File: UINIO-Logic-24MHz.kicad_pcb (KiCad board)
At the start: 2 copper layers, 48.8 x 25.5 mm, 51 parts, among them J1 Conn_01x10_Male, U1 AT24CS64-XHM, U2 74HC245C, U3 ME6211C33M5G-N, U4 CY7C68013A-56LTX, Y1 24MHz

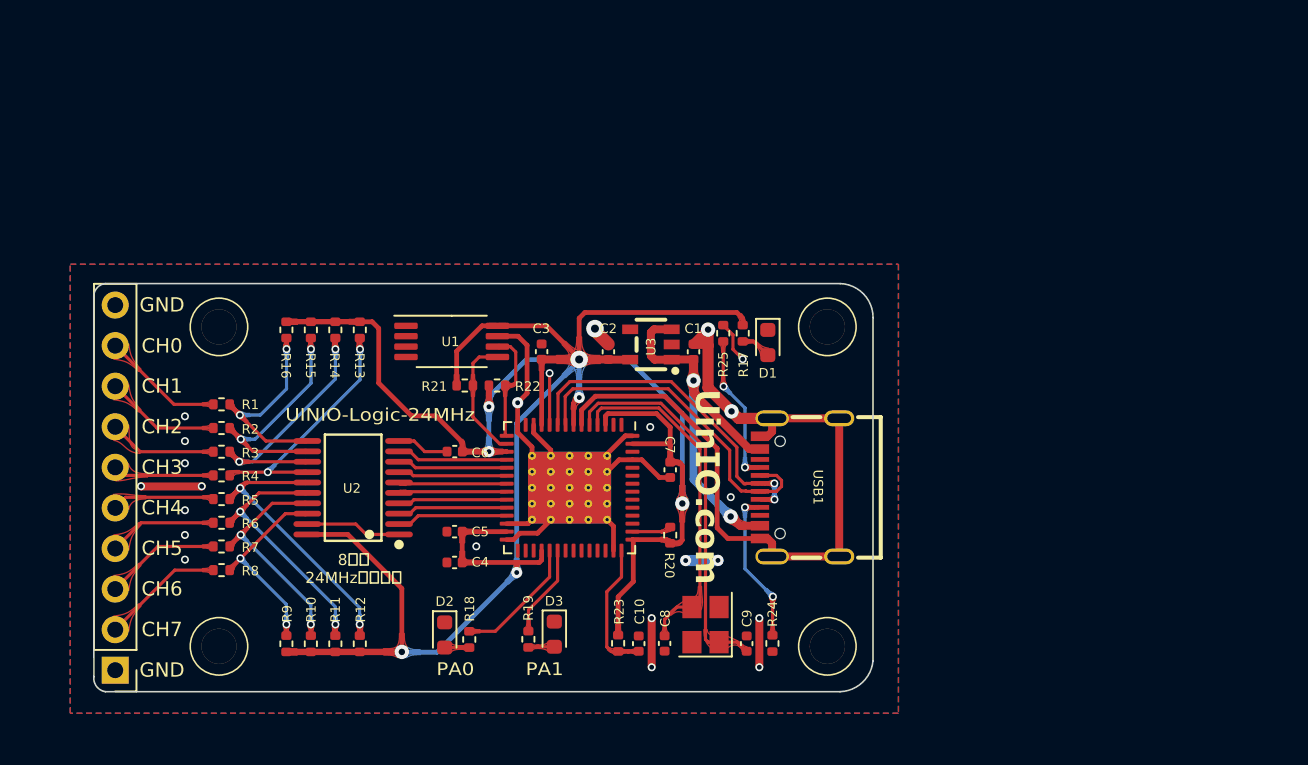
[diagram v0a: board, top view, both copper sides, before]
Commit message: Prepare version 3.1.0.
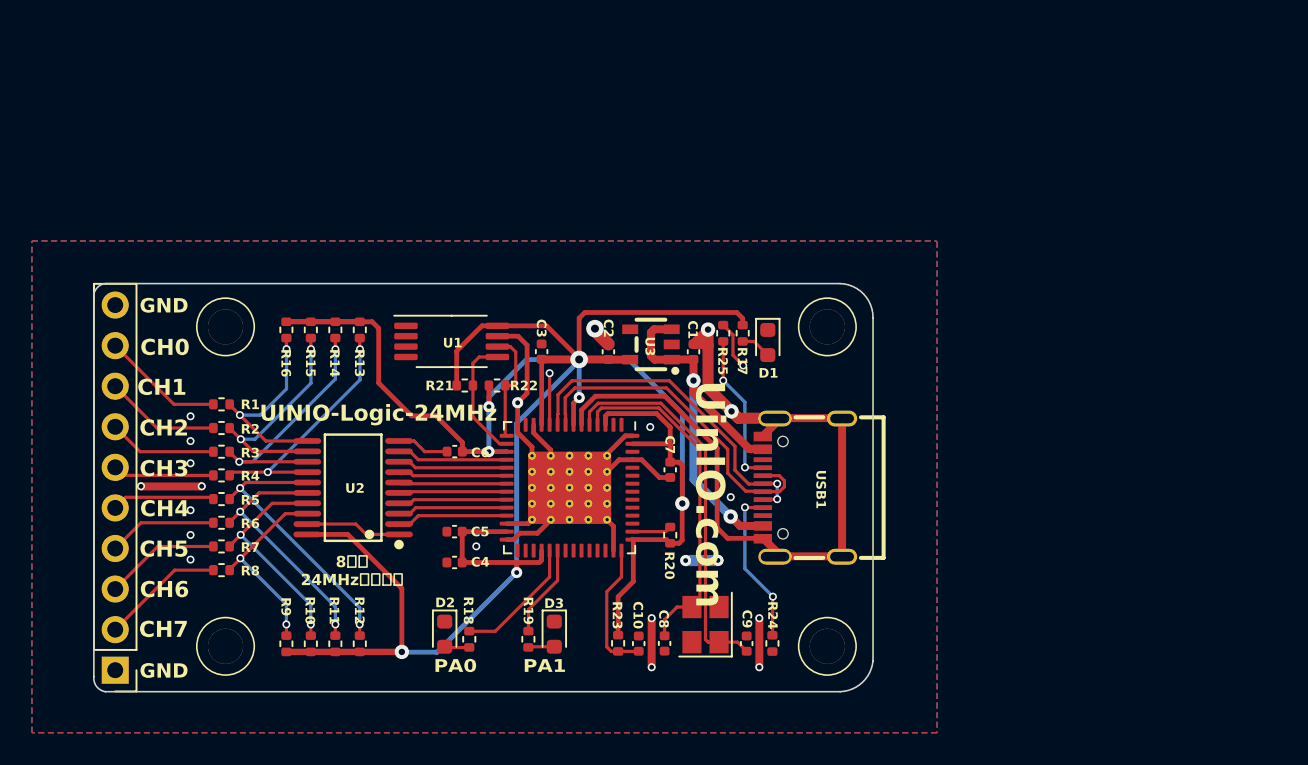
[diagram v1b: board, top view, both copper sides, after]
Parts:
- removed the ? at (144.7, 118.7)
- removed the ? at (130.6, 118.6)
- added ?: LOGO, LOGO, B.Cu at (136.1, 118.8)
- added ?: LOGO, LOGO, B.Cu at (120.4, 118.8)
- J1: value Conn_01x10_Male -> Conn_01x10_Pin
- moved HOLE1 0.41 mm to (114.5, 108.7)
- moved HOLE2 0.41 mm to (114.5, 128.7)
- moved USB1 0.18 mm to (150.6, 118.8)
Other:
- board text added: "UinIO.com"
- board text added: "Version 3.1.0"
- board text removed: "Version 3.0.0"

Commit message: Release UINIO-Logic-24MHz version 3.1.0.
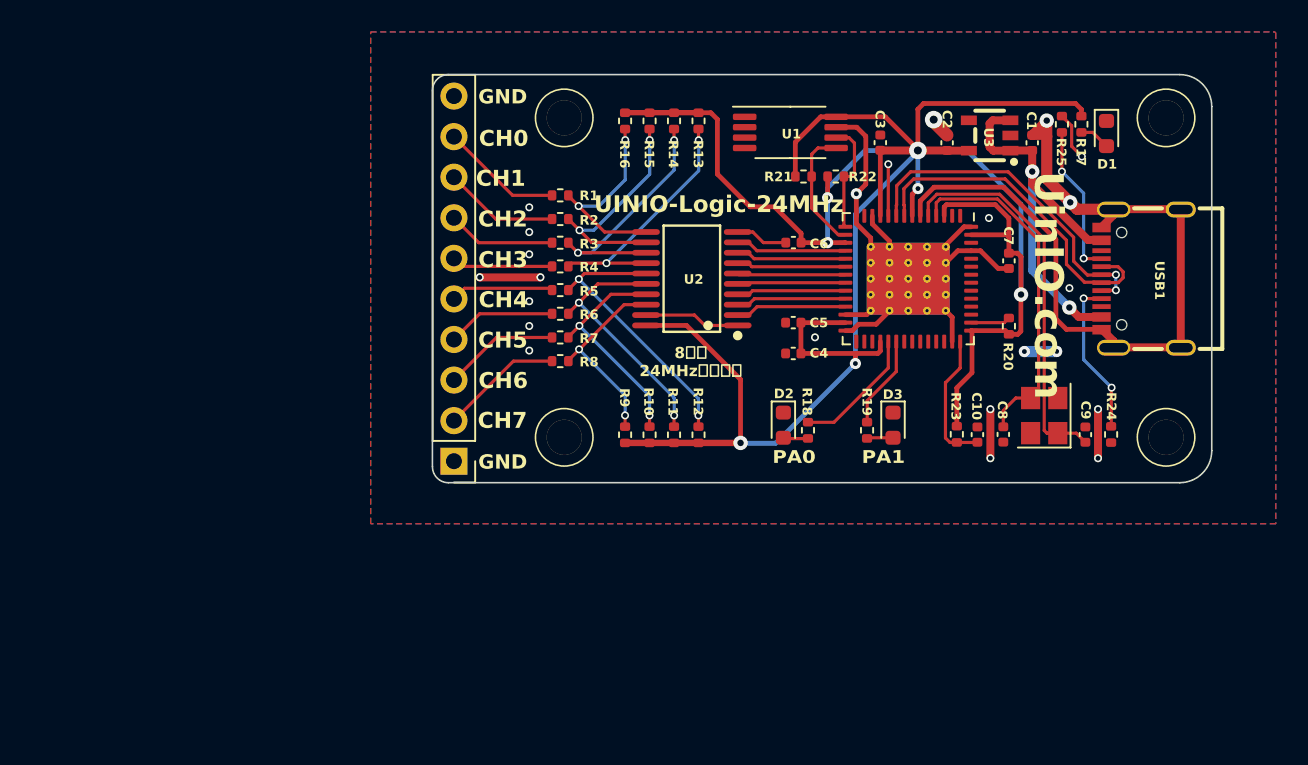
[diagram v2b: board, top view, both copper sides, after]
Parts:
- moved C1 24.9 mm to (165.0, 97.2)
- moved C10 24.9 mm to (161.6, 115.4)
- moved C8 24.9 mm to (163.2, 115.4)
- moved D1 24.9 mm to (169.7, 96.6)
- moved HOLE3 24.9 mm to (173.4, 95.6)
- moved R21 24.9 mm to (150.7, 99.3)
- moved R24 24.9 mm to (170.0, 115.4)
- moved U3 24.9 mm to (162.4, 96.7)
- moved Y1 24.9 mm to (165.8, 114.3)
- moved D3 24.9 mm to (156.3, 114.9)
- moved HOLE4 24.9 mm to (173.4, 115.6)
- moved R11 24.9 mm to (142.6, 115.5)
- moved R18 24.9 mm to (151.0, 115.2)
- moved R19 24.9 mm to (154.7, 115.2)
- moved R23 24.9 mm to (160.3, 115.4)
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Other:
- outline, holes or cut-outs redrawn
